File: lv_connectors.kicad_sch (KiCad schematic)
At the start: 34 parts, among them J10 Conn_01x10, J2 Conn_01x04, J3 Conn_01x04, J4 Conn_01x04, J6 Conn_01x02, J7 Conn_01x04, J9 Conn_01x02, Q2 NMOS, Q3 NMOS, Q4 NMOS, U15 ADP121-AUJZ33R7, U2 L7805

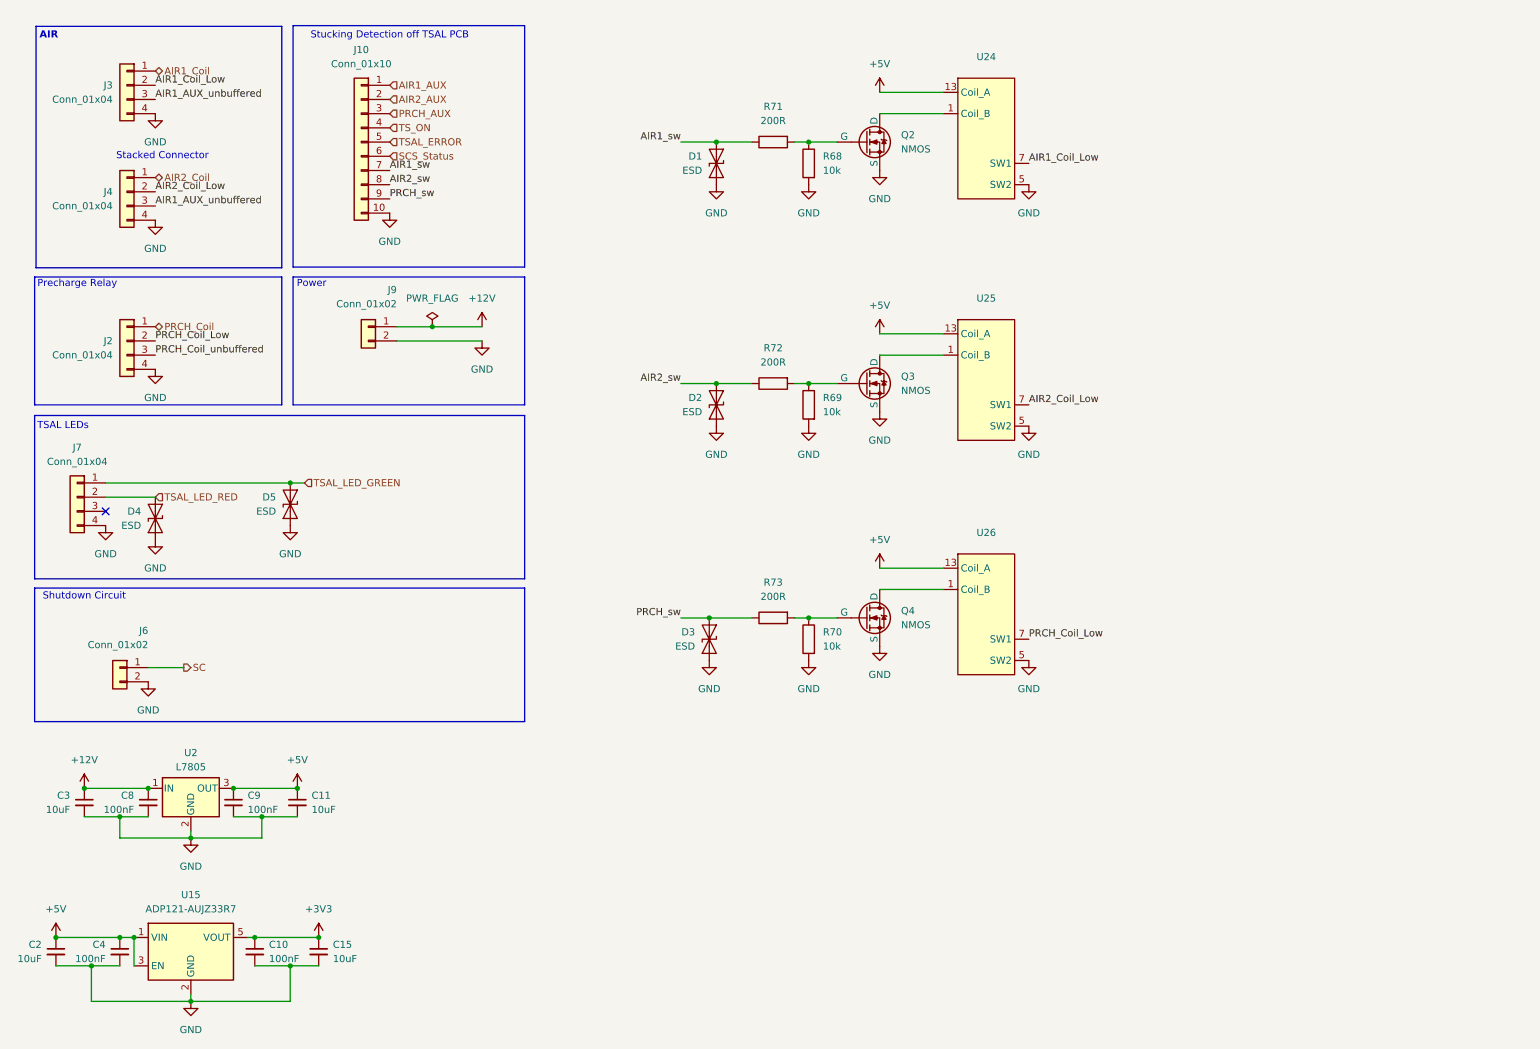
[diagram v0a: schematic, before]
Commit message: Added Rules
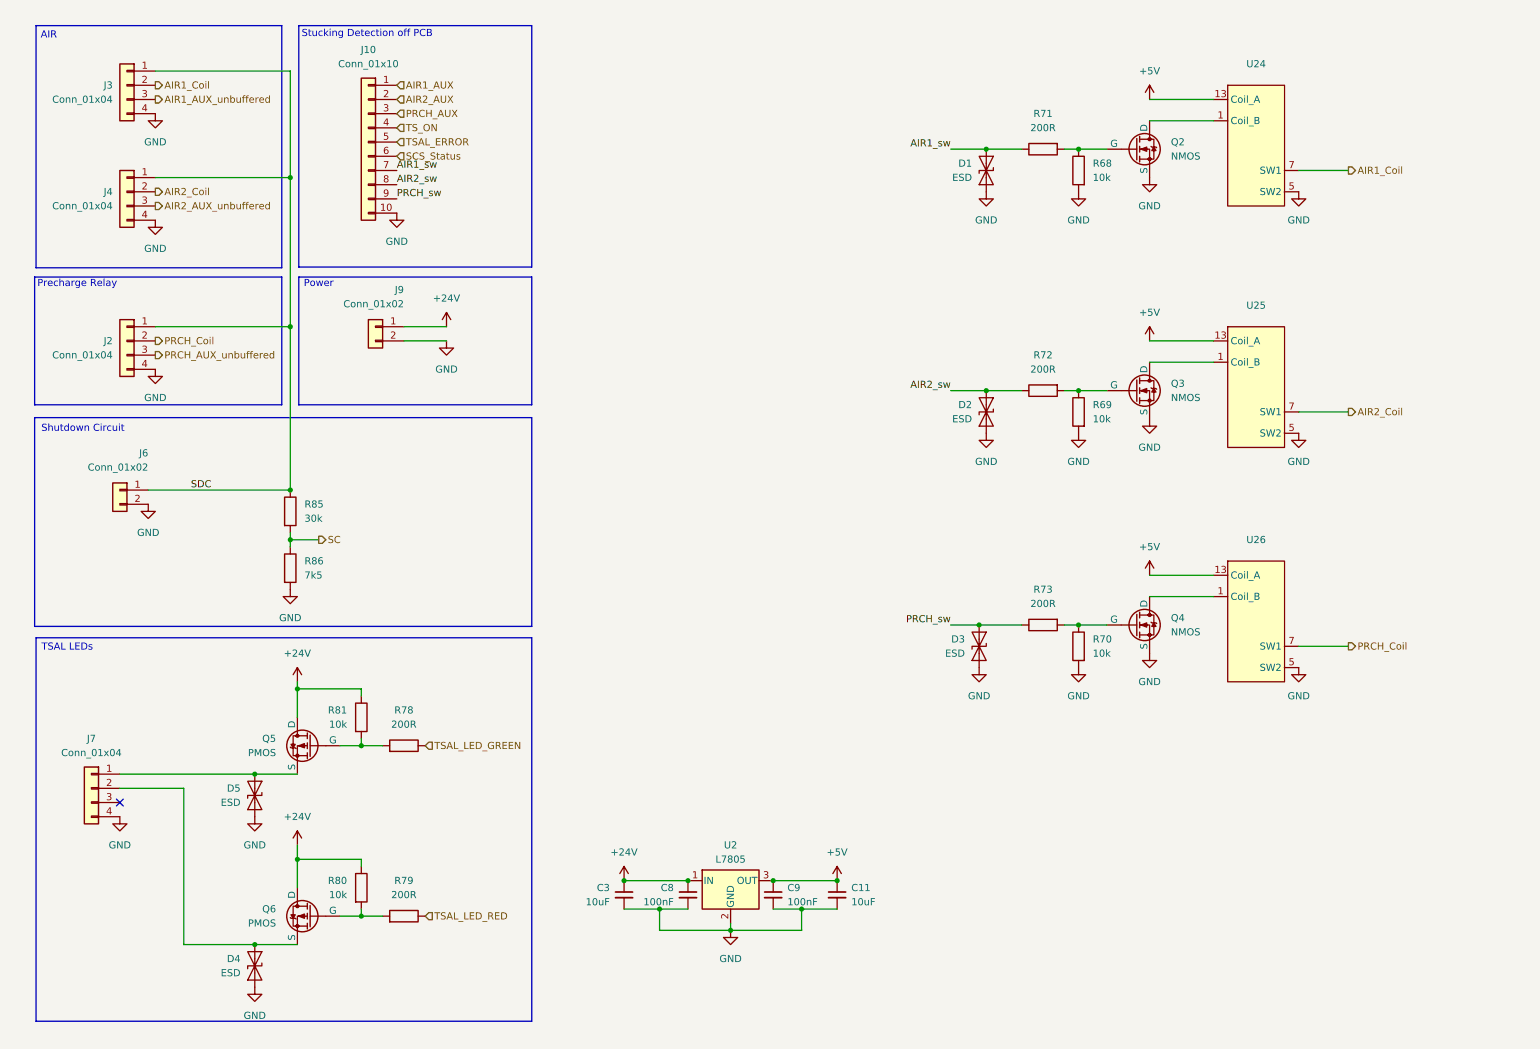
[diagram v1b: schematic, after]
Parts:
- removed C10, C4: 100nF, Capacitor_SMD:C_0603_1608Metric, symbol Device:C_Small
- removed C15, C2: 10uF, Capacitor_SMD:C_0603_1608Metric, symbol Device:C_Small
- removed U15: ADP121-AUJZ33R7, Package_TO_SOT_SMD:TSOT-23-5, symbol Regulator_Linear:ADP7142AUJZ-3.3
- added Q5, Q6: PMOS, symbol Simulation_SPICE:PMOS
- added R78, R79: 200R, symbol Device:R
- added R80, R81: 10k, symbol Device:R
- added R85: 30k, symbol Device:R
- added R86: 7k5, symbol Device:R
- U2: Cost 0,958 -> 0,949; Mouser 511-L7805ACD2T-TR -> 511-L7805ABD2T-TR
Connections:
- net AIR1_Coil_Low is gone; now on net AIR1_Coil: J3.2 (Pin_2), U24.7 (SW1)
- net AIR2_Coil_Low is gone; now on net AIR2_Coil: J4.2 (Pin_2), U25.7 (SW1)
- net PRCH_Coil_Low is gone; now on net PRCH_Coil: J2.2 (Pin_2), U26.7 (SW1)
- net AIR1_AUX_unbuffered: no longer J4.3 (Pin_3)
- net AIR1_Coil: no longer J3.1 (Pin_1)
- net AIR2_Coil: no longer J4.1 (Pin_1)
- net GND: now also R86.2
- net PRCH_Coil: no longer J2.1 (Pin_1)
- net SC: now also R85.2, R86.1; no longer J6.1 (Pin_1)
- net TSAL_LED_GREEN: now also R78.1; no longer D5.2 (A2), J7.1 (Pin_1)
- net TSAL_LED_RED: now also R79.1; no longer D4.2 (A2), J7.2 (Pin_2)
- net +12V renamed +24V
- net +24V: now also Q5.1 (D), Q6.1 (D), R80.1, R81.1
- net PRCH_Coil_unbuffered renamed PRCH_AUX_unbuffered
- new net: Q5.2 (G), R78.2, R81.2
- new net: D4.2 (A2), J7.2 (Pin_2), Q6.3 (S)
- new net: D5.2 (A2), J7.1 (Pin_1), Q5.3 (S)
- new net: Q6.2 (G), R79.2, R80.2
- new net AIR2_AUX_unbuffered: J4.3 (Pin_3)
- new net SDC: J2.1 (Pin_1), J3.1 (Pin_1), J4.1 (Pin_1), J6.1 (Pin_1), R85.1
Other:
- note added: "Stucking Detection off PCB"
- note removed: "Stacked Connector"
- note removed: "Stucking Detection off TSAL PCB"
- moved on the sheet: C11, C3, C8, C9, D1, D2, D3, D5, J10, J6, J7, J9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

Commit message: Submission Ready. ESF 15.07.24
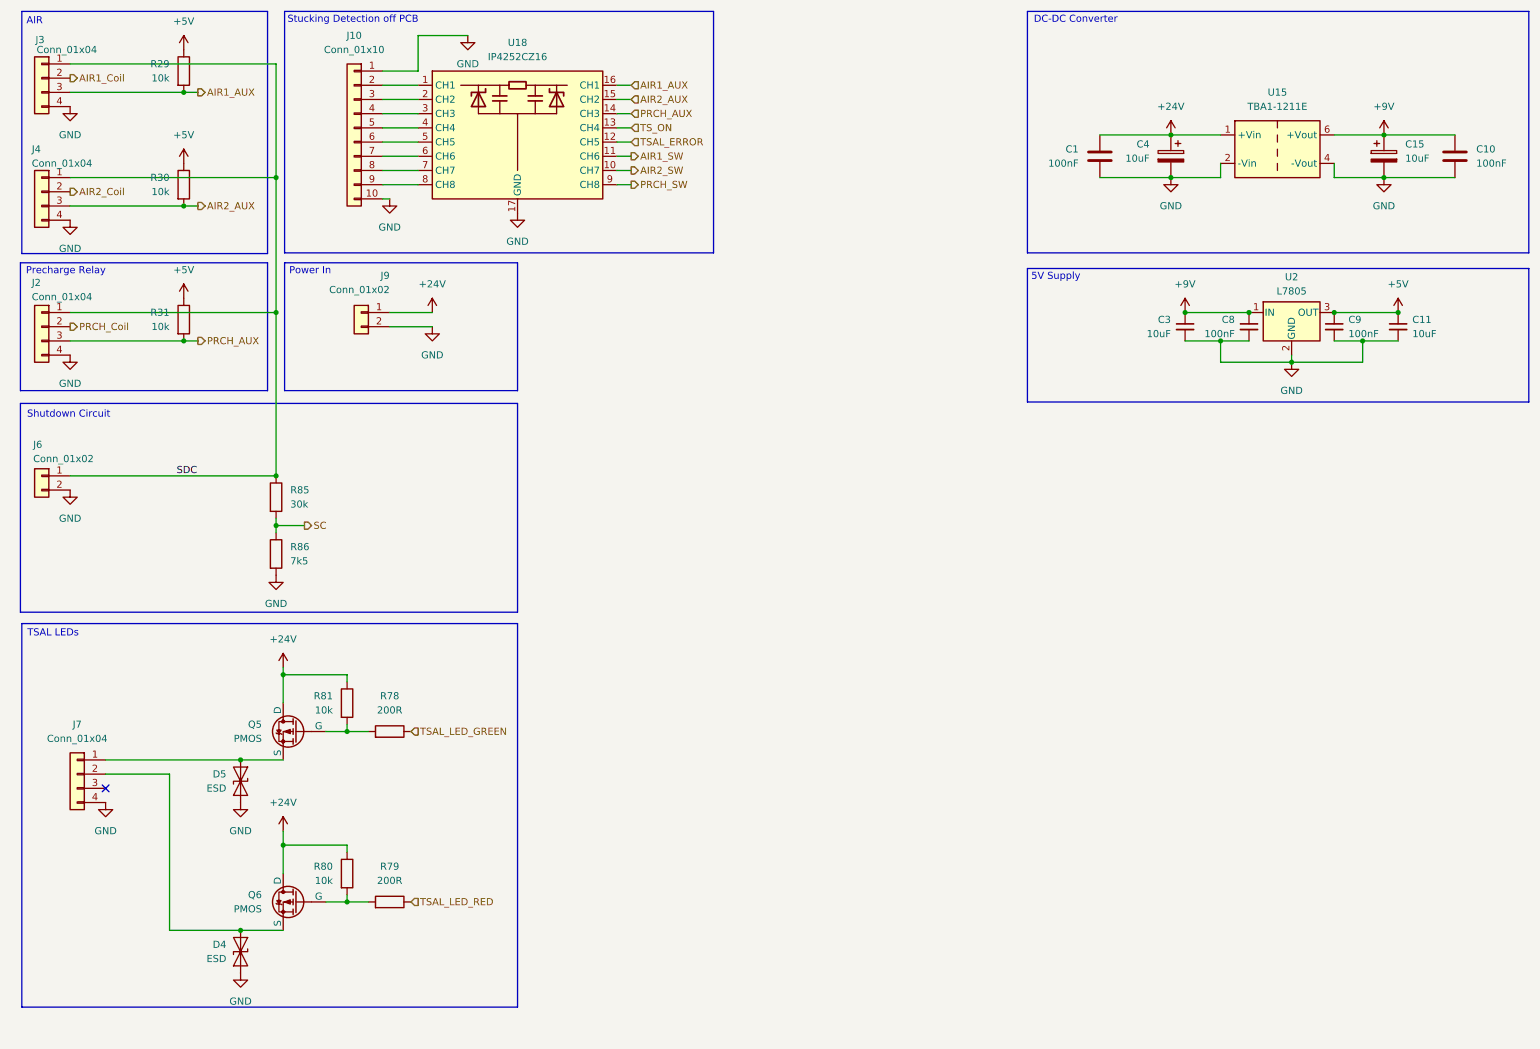
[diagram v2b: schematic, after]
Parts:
- removed D1, D2, D3: ESD, Diode_SMD:Infineon_SG-WLL-2-3_0.58x0.28_P0.36mm, symbol Diode:ESD131-B1-W0201
- removed Q2, Q3, Q4: NMOS, symbol Simulation_SPICE:NMOS
- removed R68, R69, R70: 10k, symbol Device:R
- removed R71, R72, R73: 200R, symbol Device:R
- removed U24, U25, U26: ~, symbol Zettler:AZ9371
- added C1, C10: 100nF, symbol Device:C
- added C15, C4: 10uF, symbol Device:C_Polarized
- added R29, R30, R31: 10k, symbol Device:R
- added U15: TBA1-1211E, Converter_DCDC:Converter_DCDC_TRACO_TBA1-xxxxE_Single_THT, symbol Converter_DCDC:TBA1-1211E
- added U18: IP4252CZ16, Package_SON:Nexperia_HUSON-16_USON-16-1EP_1.35x3.3mm_P0.4mm_EP0.4x2.8mm, symbol Power_Protection:IP4252CZ16
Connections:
- net AIR1_AUX_unbuffered is gone; now on net AIR1_AUX: J3.3 (Pin_3)
- net AIR2_AUX_unbuffered is gone; now on net AIR2_AUX: J4.3 (Pin_3)
- net PRCH_AUX_unbuffered is gone; now on net PRCH_AUX: J2.3 (Pin_3)
- net +24V: now also C1.1, C4.1, U15.1 (+Vin); no longer C3.1, C8.1, U2.1 (IN)
- net +5V: now also R29.1, R30.1, R31.1
- net AIR1_AUX: now also R29.2, U18.16 (CH1); no longer J10.1 (Pin_1)
- net AIR2_AUX: now also R30.2, U18.15 (CH2); no longer J10.2 (Pin_2)
- net GND: now also J10.1 (Pin_1), C1.2, C10.2, C15.2, C4.2, U15.2 (-Vin), U15.4 (-Vout), U18.17 (GND)
- net PRCH_AUX: now also R31.2, U18.14 (CH3); no longer J10.3 (Pin_3)
- net TSAL_ERROR: now also U18.12 (CH5); no longer J10.5 (Pin_5)
- net TS_ON: now also U18.13 (CH4); no longer J10.4 (Pin_4)
- net AIR1_sw: no longer names the net of J10.7 (Pin_7)
- net AIR1_sw: now also U18.6 (CH6)
- net AIR2_sw: no longer names the net of J10.8 (Pin_8)
- net AIR2_sw: now also U18.7 (CH7)
- net PRCH_sw: no longer names the net of J10.9 (Pin_9)
- net PRCH_sw: now also U18.8 (CH8)
- net SCS_Status: no longer names the net of J10.6 (Pin_6)
- net SCS_Status: now also U18.5 (CH5)
- new net: J10.2 (Pin_2), U18.1 (CH1)
- new net: J10.3 (Pin_3), U18.2 (CH2)
- new net: J10.4 (Pin_4), U18.3 (CH3)
- new net: J10.5 (Pin_5), U18.4 (CH4)
- new net +9V: C10.1, C15.1, C3.1, C8.1, U15.6 (+Vout), U2.1 (IN)
- new net AIR1_SW: U18.11 (CH6)
- new net AIR2_SW: U18.10 (CH7)
- new net PRCH_SW: U18.9 (CH8)
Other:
- note added: "5V Supply"
- note added: "DC-DC Converter"
- note added: "Power In"
- note removed: "Power"
- moved on the sheet: C11, C3, C8, C9, D4, D5, J10, J2, J3, J4, J6, J7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

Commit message: ⠀⠀⠀⠀⠀⠀⠀⠀⠀⠀⠀⠀⠀⠀⠀⠀⠀⠀⠀⠀⠀⠀⠀⠀⠀⠀⠀⠀⠀⠀⠀⠀⠀⠀⠀⠀⠀⣠⣤⣤⣤⡀⠀⠀⠀⠀⠀⠀⠀⠀⠀⠀⠀⠀⠀⠀⠀⠀⠀⠀⠀⠀⠀⠀⠀ ⠀⠀⠀⠀⠀⠀⠀⠀⠀⠀⠀⠀⠀⠀⠀⠀⠀⠀⠀⠀⠀⠀⠀⠀⠀⠀⠀⠀⠀⠀⠀⠀⠀⠀⣠⣶⣿⠟⠉⠉⠻⣿⡄⠀⠀⠀⠀⠀⠀⠀⠀⠀⠀⠀⠀⠀⠀⠀⠀⠀⠀⠀⠀⠀⠀ ⠀⠀⠀⠀⠀⠀⠀⠀⠀⠀⠀⠀⠀⠀⠀⠀⠀⠀⠀⠀⠀⠀⠀⠀⠀⠀⠀⠀⠀⠀⠀⢀⣤⣾⠿⠉⠀⠀⠀⠀⠀⠹⣿⡄⠀⠀⠀⠀⠀⠀⠀⠀⠀⠀⠀⠀⠀⠀⠀⠀⠀⠀⣀⣴⣾ ⠀⠀⠀⠀⠀⠀⠀⠀⠀⠀⠀⠀⠀⠀⠀⠀⠀⠀⠀⠀⠀⠀⠀⠀⠀⠀⠀⠀⠀⢀⣴⣿⠟⠁⠀⠀⠀⠀⠀⠀⠀⠀⣿⣿⠀⠀⠀⠀⠀⠀⠀⠀⠀⠀⠀⠀⠀⠀⠀⣀⣴⣾⡿⠛⠉ ⠀⠀⠀⠀⠀⠀⠀⠀⠀⠀⠀⠀⠀⠀⠀⠀⠀⠀⠀⠀⠀⠀⠀⠀⠀⠀⠀⢀⣴⣿⠟⠁⠀⠀⠀⠀⠀⠀⠀⠀⠀⠀⢸⣿⡆⠀⠀⠀⠀⠀⠀⠀⠀⠀⠀⠀⢀⣴⣾⡿⠟⠁⠀⠀⠀ ⠀⠀⠀⠀⠀⠀⠀⠀⠀⠀⠀⠀⠀⠀⠀⠀⠀⠀⠀⠀⠀⠀⠀⠀⢀⣀⣴⣿⡿⠃⠀⠀⠀⠀⠀⠀⠀⠀⠀⠀⠀⠀⢸⣿⣷⣶⣶⣦⣤⣤⣄⡀⠀⢀⣠⣾⣿⠿⠋⠀⠀⠀⠀⠀⣠ ⠀⠀⠀⠀⠀⠀⠀⠀⠀⠀⠀⠀⠀⠀⠀⠀⠀⠀⠀⠀⠀⠀⠀⣼⣿⣿⡿⠋⠀⠀⠀⠀⠀⠀⠀⠀⠀⠀⠀⣠⣤⠶⠞⣿⠟⠋⠉⠉⠙⣻⠿⢿⣿⣿⣿⠟⠁⠀⠀⠀⠀⠀⢀⡼⠁ ⠀⠀⠀⠀⠀⠀⠀⠀⠀⠀⠀⠀⠀⠀⠀⠀⠀⠀⠀⠀⠀⠀⢰⣿⠁⠛⠀⠀⠀⠀⠀⠀⠀⠀⠀⠀⠀⠀⣰⠟⠁⢠⡞⠁⠀⠀⠀⢀⡴⠋⠀⢀⡿⠋⠁⠀⠀⠀⠀⠀⠀⠀⡞⠁⠀ ⠀⠀⠀⠀⠀⠀⠀⠀⠀⠀⠀⠀⠀⠀⠀⠀⠀⠀⠀⠀⠀⣠⣼⣿⡄⠀⠀⠀⠀⠀⠀⠀⠀⠀⠀⠀⠀⣼⠃⠀⢠⠏⠀⠀⠀⠀⣰⠏⠀⠀⣠⠟⠀⠀⠀⠀⠀⠀⠀⠀⠀⢸⡥⠤⡀ ⠀⠀⠀⠀⠀⠀⠀⠀⠀⠀⠀⠀⠀⠀⠀⠀⠀⠀⠀⠀⣰⣿⠟⠁⠀⠀⠀⠀⠀⠀⠀⠀⠀⠀⠀⠀⠠⣇⠀⣠⡏⠀⠀⠀⠀⣼⠁⠀⠀⣰⠋⠀⠀⠀⠀⠀⠀⠀⠀⠀⠀⠀⢀⡴⠁ ⠀⠀⠀⠀⠀⠀⠀⠀⠀⠀⠀⠀⠀⠀⠀⠀⣀⣄⣄⣼⣿⠋⠀⠀⠀⠀⠀⠀⠀⠀⠀⠀⠀⠀⠀⠀⠀⢻⡶⠋⠀⠀⠀⠀⢸⣧⠀⠀⣴⠃⠀⠀⠀⠀⠀⠀⠀⠀⠀⠀⠀⠀⠘⢧⠀ ⠀⠀⠀⠀⠀⠀⠀⠀⢀⣀⣀⠀⠀⠀⠀⣾⡿⠿⣿⡿⠁⠀⠀⠀⠀⠀⠀⣠⣶⣶⣶⡀⠀⠀⠀⠀⠀⠀⠀⠀⠀⠀⠀⠀⠀⠙⠛⠛⠁⠀⠀⠀⠀⠀⠀⠀⠀⠀⠀⠀⠀⠀⠀⠈⠳ ⠀⠀⠀⠀⠀⠀⢀⣾⠿⠛⢿⣿⣷⣄⡀⣿⠃⠀⠈⠀⠀⠀⠀⠀⠀⢀⣾⣿⣿⣿⣿⣧⠀⠀⠀⠀⠀⠀⠀⠀⠀⠀⠀⠀⠀⠀⠀⠀⠀⠀⠀⠀⠀⠀⠀⠀⠀⠀⠀⠀⠀⠀⠀⠀⠀ ⠀⠀⠀⣠⣤⣦⣼⣿⠀⠀⠀⣿⣿⣿⣿⣿⣦⣀⠀⠀⠀⠀⠀⠀⠀⣿⣿⣿⣿⣿⣿⡿⠀⠀⠀⢀⣀⣀⣀⣀⡀⠀⠀⠀⠀⠀⠀⠀⠀⠀⠀⣤⣾⣿⣿⣿⣷⣄⠀⠀⠀⠀⠀⠀⠀ ⠀⣠⣾⡿⠋⠉⠉⠁⠀⠀⠀⠀⠉⢯⡙⠻⣿⣿⣷⣤⡀⠀⠀⠀⠀⢿⣿⣿⣿⣿⡿⠃⢀⡤⠖⠋⠉⠉⠉⠉⠉⠉⠒⠦⣄⠀⠀⠀⠀⠀⣾⣿⣿⣿⣿⣿⣿⣿⣧⠀⠀⠀⠀⠀⠀ ⣾⣿⠋⠀⠀⠀⠀⣀⣀⠀⠀⠀⠀⠀⠙⢦⣄⠉⠻⢿⣿⣷⣦⡀⠀⠈⠙⠛⠛⠋⠀⢰⠟⡇⠀⠀⠀⠀⠀⠀⠀⠀⠀⠀⠈⠳⣄⠀⠀⠀⣿⣿⣿⣿⣿⣿⣿⣿⣿⠀⠀⠀⠀⠀⠀ ⣿⡇⠀⠀⠀⣴⠟⣫⣿⣿⣄⠀⠀⠀⠀⡶⢌⡙⠶⣤⡈⠛⠿⣿⣷⣦⣀⠀⠀⠀⠀⡇⠀⢻⣄⠀⠀⣠⢷⠀⠀⠀⠀⠀⡶⠀⠘⡆⠀⠀⠻⣿⣿⣿⣿⣿⣿⣿⡟⠀⠀⠀⠀⠀⠀ ⣿⡇⠀⠀⢸⣟⢸⣿⣿⣿⣿⠀⠀⠀⠀⡇⠀⠈⠛⠦⣝⡳⢤⣈⠛⠻⣿⣷⣦⣀⠀⠀⠀⠀⠈⠙⠋⠁⠀⠛⠦⠤⠤⠚⠁⠀⠀⢳⠀⠀⠀⠈⠛⠿⠿⠿⠟⠋⠀⠀⠀⠀⠀⠀⠀ ⣿⡇⠀⠀⠈⢿⣞⣿⣿⣿⠏⠀⠀⠀⠀⡇⠀⠀⠀⠀⠀⠙⠳⢬⣛⠦⠀⠙⢻⣿⣷⣦⣀⠀⠀⠀⠀⠀⠀⠀⠀⠀⠀⠀⠀⠀⠀⡞⠀⠀⠀⠀⠀⠀⠀⠀⠀⠀⠀⠀⠀⠀⠀⠀⠀ ⣿⡇⠀⠀⠀⠀⠉⠛⠋⠁⠀⠀⠀⠀⠀⡇⠀⠀⠀⠀⠀⠀⠀⠀⠈⠁⠀⠀⠈⣿⠉⢻⣿⣷⣦⣀⠀⠀⠀⠀⠀⠀⠀⠀⠀⢀⡼⠁⠀⠀⠀⠀⠀⠀⠀⠀⠀⠀⠀⠀⠀⠀⠀⠀⠀ ⣿⡇⠀⠀⠀⠀⠀⣠⣄⠀⠀⢰⠶⠒⠒⢧⣄⡀⠀⠀⠀⠀⠀⠀⠀⠀⠀⠀⠀⣿⠀⢸⡇⢸⡟⢿⣷⣦⣴⣶⣶⣶⣶⣤⣔⠋⠀⠀⠀⠀⠀⠀⠀⠀⠀⠀⠀⠀⠀⠀⠀⠀⠀⠀⠀ ⣿⡇⠀⠀⣤⠀⠀⠿⠿⠁⢀⡿⠀⠀⠀⡄⠈⠙⡷⢦⣄⡀⠀⠀⠀⠀⠀⠀⠀⣿⠀⢸⡇⢸⡇⠀⣿⠙⣿⣿⣉⠉⠙⠿⣿⣧⠀⠀⠀⠀⠀⠀⠀⠀⠀⠀⠀⠀⠀⠀⠀⠀⠀⠀⠀ ⣿⡇⠀⠀⠙⠷⢤⣀⣠⠴⠛⠁⠀⠀⠀⠇⠀⠀⡇⢸⡏⢹⡷⢦⣄⡀⠀⠀⠀⣿⡀⢸⡇⢸⡇⠀⡟⠀⢸⠀⢹⡷⢦⣄⣘⣿⡆⠀⠀⠀⠀⠀⠀⠀⠀⠀⠀⠀⠀⠀⠀⠀⠀⠀⠀ ⣿⣿⠢⣤⡀⠀⠀⠀⠀⠀⠀⣠⠾⣿⣿⡷⣤⣀⡇⠸⡇⢸⡇⢸⠉⠙⠳⢦⣄⡻⢿⣾⣧⣸⣧⠀⡇⠀⢸⠀⢸⡇⢤⣈⠙⠻⣿⣆⠀⠀⠀⠀⠀⠀⠀⠀⠀⠀⠀⠀⠀⠀⠀⠀⠀ ⢹⣿⣷⣌⡉⠛⠲⢶⣶⠖⠛⠛⢶⣄⡉⠛⠿⣽⣿⣶⣧⣸⡇⢸⠀⠀⠀⠀⠈⠙⠲⢮⣝⠻⣿⣷⣷⣄⣸⠀⢸⡇⠀⠈⠁⠀⢸⣿⠀⠀⠀⠀⠀⠀⠀⠀⠀⠀⠀⠀⠀⠀⠀⠀⠀ ⠀⠈⠙⠻⢿⣷⣶⣤⣉⡻⢶⣄⣀⠈⠙⠳⢦⣈⡉⠻⢿⣿⣷⣾⣦⡀⠀⠀⠀⠀⠀⠀⠈⠙⠲⢭⣛⠿⣿⣷⣼⡇⠀⠀⠀⠀⠈⣿⡇⠀⠀⠀⠀⠀⠀⣀⠀⠀⠀⠀⠀⠀⠀⠀⣀ ⠀⠀⠀⠀⠀⠈⠙⠻⢿⣿⣷⣶⣽⣻⡦⠀⠀⠈⠙⠷⣦⣌⡙⠻⢿⣟⣷⣤⣀⠀⠀⠀⠀⠀⠀⠀⠈⠙⠳⢯⣻⡇⠀⠀⠀⠀⠀⢸⣿⠀⣀⠀⠀⠀⠀⠈⠳⣄⠀⠀⠀⢀⡏⠙⠛ ⠀⠀⠀⠀⠀⠀⠀⠀⠀⠈⠛⠻⢿⣿⣿⣿⣶⣤⣤⣤⣀⣈⠛⠷⣤⣈⡛⠷⢽⡻⢶⣄⣀⠀⠀⠀⠀⠀⠀⠀⠈⠛⠳⢤⣀⠀⠀⢸⣿⡀⠈⠳⢤⣀⣀⣰⠃⠈⠛⠶⠶⠿⠃⠀⠀ ⠀⠀⠀⠀⠀⠀⠀⠀⠀⠀⠀⠀⠀⢈⣿⡿⠛⠉⠙⠛⠛⠻⢷⣦⣄⣩⣿⠶⠖⠛⠛⠛⠛⠛⠛⠿⢷⣶⣦⣄⠀⠀⠀⠀⠉⢻⣶⣿⣿⠇⠀⠀⠀⠉⠉⠀⠀⠀⠀⠀⠀⠀⠀⠀⠀ ⠀⠀⠀⠀⠀⠀⠀⠀⠀⠀⠀⠀⠀⣼⣿⠁⠀⠀⠀⠀⠀⠀⠀⣿⣿⠋⠀⠀⠀⠀⠀⣠⠖⠂⠀⠀⠀⠈⠙⠿⣿⣦⡄⠀⠀⣸⣿⠟⠋⠀⠀⠀⠀⠀⠀⠀⠀⠀⠀⠀⠀⠀⠀⠀⠀ ⠀⠀⠀⠀⠀⠀⠀⠀⠀⠀⠀⠀⢰⣿⡟⠀⠀⠀⠀⠀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
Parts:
- C1, C10, C15, C4: footprint (none) -> Capacitor_SMD:C_0603_1608Metric
- Q5, Q6: footprint (none) -> Package_TO_SOT_SMD:SOT-23-3
- R29, R30, R31, R78, R79, R80, R81, R85, R86: footprint (none) -> Resistor_SMD:R_0603_1608Metric
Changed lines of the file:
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@@
 			)
 		)
-		(property "Footprint" ""
+		(property "Footprint" "Resistor_SMD:R_0603_1608Metric"
 			(at 80.01 144.018 90)
 			(effects
@@
 			)
 		)
-		(property "Footprint" ""
+		(property "Footprint" "Package_TO_SOT_SMD:SOT-23-3"
 			(at 58.42 170.18 0)
 			(effects
@@
 			)
 		)
+		(property "resistor datasheet" ""
+			(at 63.5 172.72 0)
+			(effects
+				(font
+					(size 1.27 1.27)
+				)
+			)
+		)
 		(pin "1"
 		)
@@
 			)
 		)
-		(property "Footprint" ""
+		(property "Footprint" "Resistor_SMD:R_0603_1608Metric"
 			(at 70.612 137.16 90)
 			(effects
@@
 			)
 		)
-		(property "Footprint" ""
+		(property "Footprint" "Capacitor_SMD:C_0603_1608Metric"
 			(at 218.7448 43.18 0)
 			(effects
@@
 			)
 		)
-		(property "Footprint" ""
+		(property "Footprint" "Capacitor_SMD:C_0603_1608Metric"
 			(at 206.0448 43.18 0)
 			(effects
@@
 			)
 		)
-		(property "Footprint" ""
+		(property "Footprint" "Resistor_SMD:R_0603_1608Metric"
 			(at 80.01 174.498 90)
 			(effects
@@
 			)
 		)
-		(property "Footprint" ""
+		(property "Footprint" "Resistor_SMD:R_0603_1608Metric"
 			(at 41.402 44.45 90)
 			(effects
@@
 			)
 		)
-		(property "Footprint" ""
+		(property "Footprint" "Capacitor_SMD:C_0603_1608Metric"
 			(at 258.7752 43.18 0)
 			(effects
@@
 			)
 		)
-		(property "Footprint" ""
+		(property "Footprint" "Resistor_SMD:R_0603_1608Metric"
 			(at 41.402 24.13 90)
 			(effects
@@
 			)
 		)
-		(property "Footprint" ""
+		(property "Footprint" "Resistor_SMD:R_0603_1608Metric"
 			(at 57.912 100.33 90)
 			(effects
@@
 			)
 		)
-		(property "Footprint" ""
+		(property "Footprint" "Resistor_SMD:R_0603_1608Metric"
 			(at 57.912 110.49 90)
 			(effects
@@
 			)
 		)
-		(property "Footprint" ""
+		(property "Footprint" "Package_TO_SOT_SMD:SOT-23-3"
 			(at 58.42 139.7 0)
 			(effects
@@
 			)
 		)
-		(property "Footprint" ""
+		(property "Footprint" "Capacitor_SMD:C_0603_1608Metric"
 			(at 271.4752 43.18 0)
 			(effects
@@
 			)
 		)
-		(property "Footprint" ""
+		(property "Footprint" "Resistor_SMD:R_0603_1608Metric"
 			(at 41.402 68.58 90)
 			(effects
@@
 			)
 		)
-		(property "Footprint" ""
+		(property "Footprint" "Resistor_SMD:R_0603_1608Metric"
 			(at 70.612 167.64 90)
 			(effects
